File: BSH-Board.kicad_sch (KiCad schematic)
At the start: 61 parts, among them J1 667101210103, J2 MICRO QTZB5.0, Q1 MMST3904, SW1 TS-3025-B-C-B, SW2 TS-3025-B-C-B, SW3 SW_DIP_x01, U1 74LVC1G07, U2 74LVC1G17, U3 AP63203WU, U4 ESP32-C6-MINI-1-N4

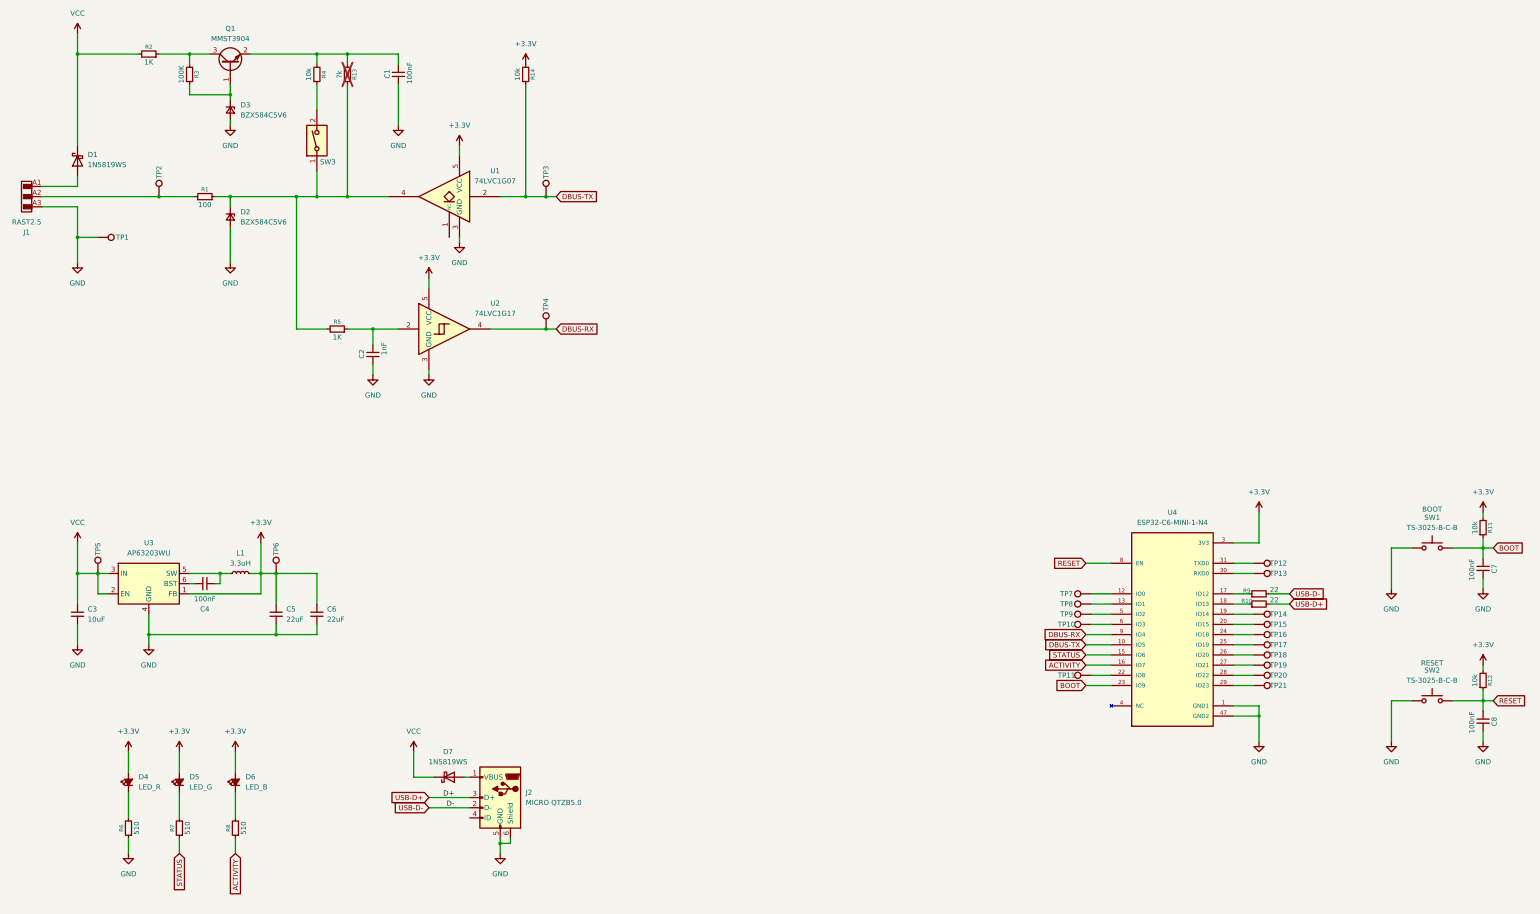
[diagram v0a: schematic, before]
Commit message: Various minor improvements
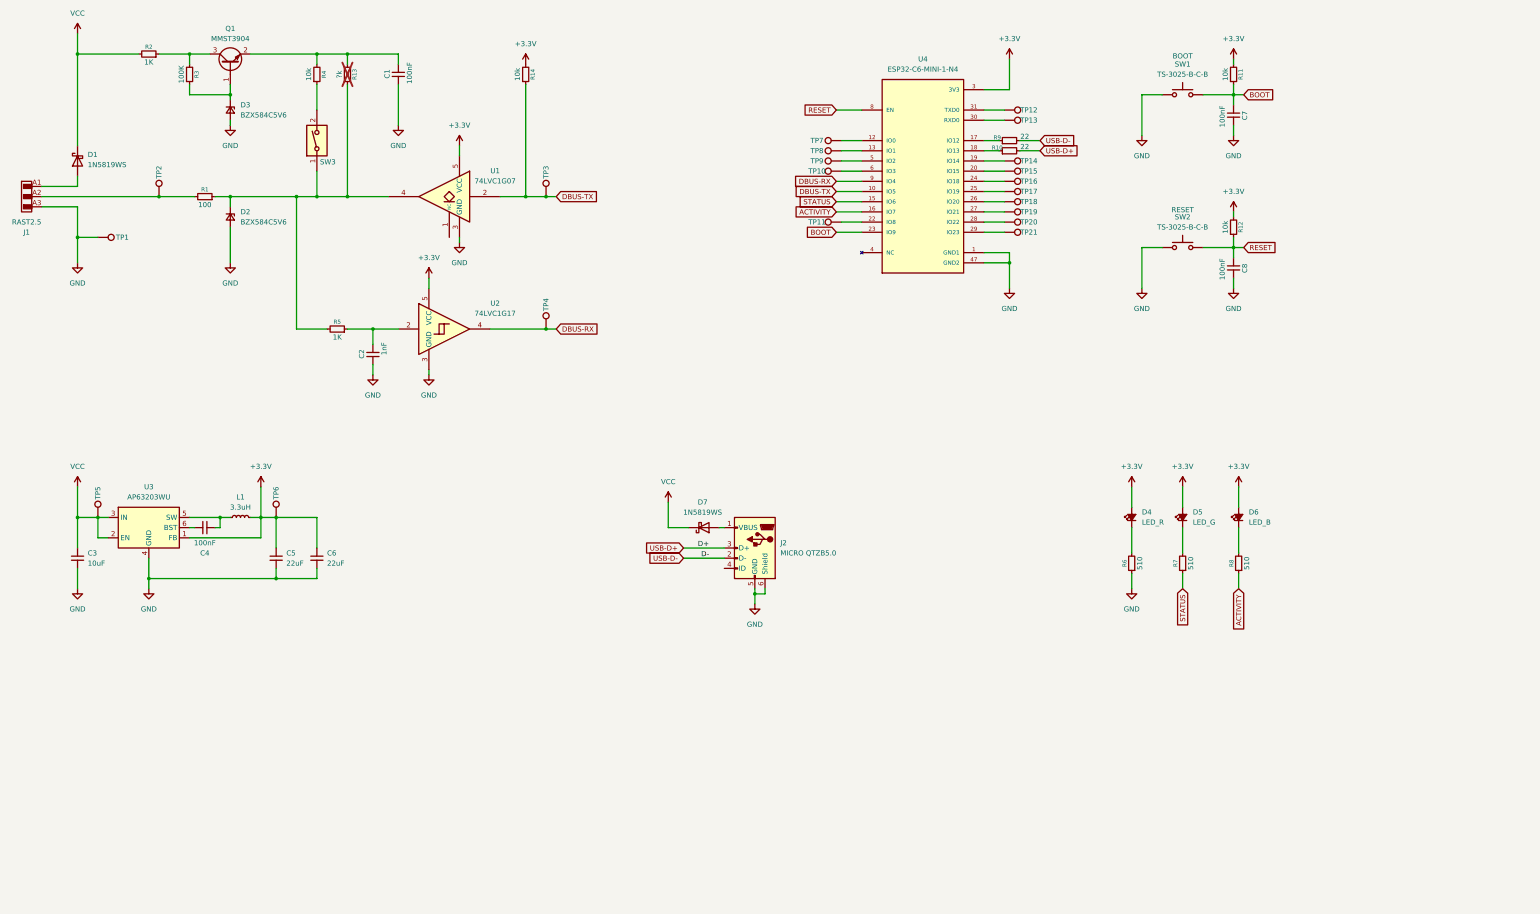
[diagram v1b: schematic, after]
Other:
- moved on the sheet: C3, C4, C5, C6, C7, C8, D4, D5, D6, D7, J2, L1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

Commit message: Hopefully fixed output now
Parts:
- SW3: LCSC (none) -> C3293141
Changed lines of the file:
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@@
+			)
+		)
+		(property "LCSC" "C3293141"
+			(at 99.06 60.96 90)
+			(effects
+				(font
+					(size 1.27 1.27)
+				)
+				(hide yes)
 			)
 		)
